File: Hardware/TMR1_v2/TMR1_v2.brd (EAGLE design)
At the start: 34.3 x 34.3 mm, 47 parts, among them U1 ATMEGA328P_TQFP, U2 MCP79410I/SN, Y1 32.768kHz

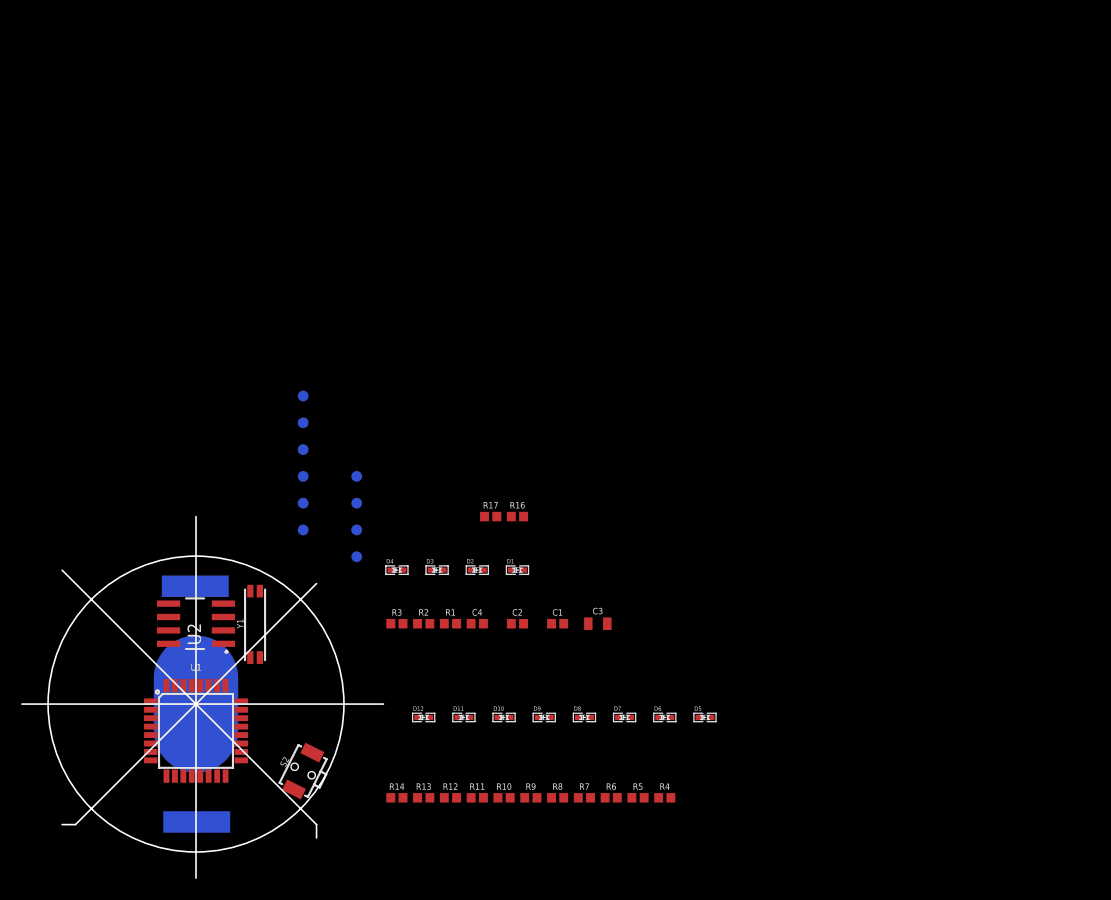
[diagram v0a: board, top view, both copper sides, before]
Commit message: std easy schematic with all elements in board before route
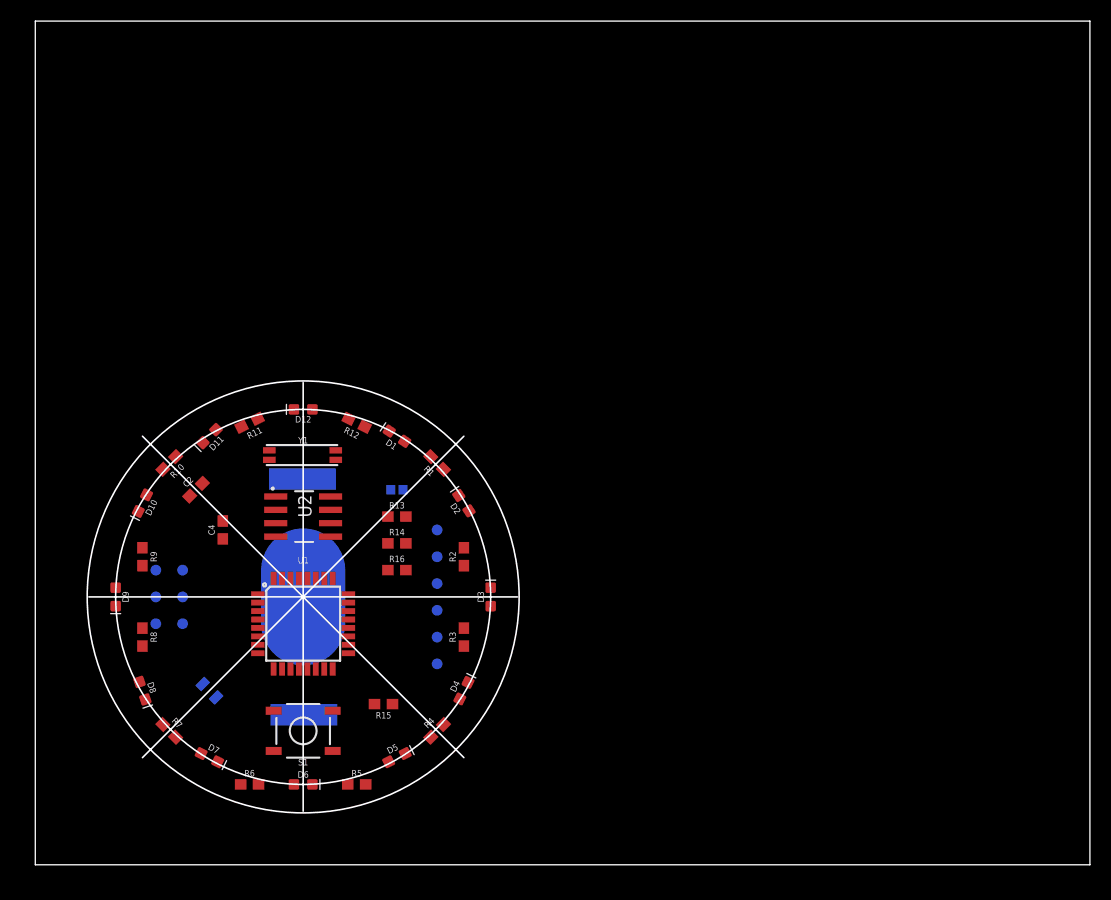
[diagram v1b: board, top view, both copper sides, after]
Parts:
- removed R17: 4.7k, SparkFun-Resistors:0402
- removed S2: MOMENTARY-SWITCH-SPST-SMD-RIGHT-ANGLE, SparkFun-Switches:TACTILE_SWITCH_SMD_RIGHT_ANGLE
- added R15: 10k, SparkFun-Resistors:0603
- added S1: MOMENTARY-SWITCH-SPST-SMD-5.2MM, SparkFun-Switches:TACTILE_SWITCH_SMD_5.2MM
- added TP11, TP12: TEST-POINT3X4, SparkFun-Connectors:PAD.03X.04
- C2, C4: value 6.8pF -> 22pF; device SparkFun-Capacitors:0402 -> SparkFun-Capacitors:0603
- C3: value 10uF -> 100nF
- D1, D10, D11, D12, D2, D3, D4, D5, D6, D7, D8, D9: device standardparts:0402.LED -> SparkFun-LED:LED-0603
- R1, R10, R11, R12, R2, R3, R4, R5, R6, R7, R8, R9: value 200 -> 330; device SparkFun-Resistors:0402 -> SparkFun-Resistors:0603
- R13, R14: device SparkFun-Resistors:0402 -> SparkFun-Resistors:0603
- R16: value 4.7k -> 10k; device SparkFun-Resistors:0402 -> SparkFun-Resistors:0603
- moved R10 44.9 mm to (12.7, 38.1), turned to 225 degrees
- moved R9 43.3 mm to (10.2, 29.2), turned to 270 degrees
- moved D9 42.2 mm to (7.62, 25.4), turned to 270 degrees
- moved R8 42.2 mm to (10.2, 21.6), turned to 270 degrees
- moved D8 42.0 mm to (10.2, 16.5), turned to 288.5 degrees
- moved R11 41.6 mm to (20.3, 41.9), turned to 206.5 degrees
- moved R7 39.9 mm to (12.7, 12.7), turned to 315 degrees
- moved D10 39.9 mm to (10.2, 34.3), turned to 243.5 degrees
- moved D7 39.6 mm to (16.5, 10.2), turned to 333.5 degrees
- moved C3 37.4 mm to (16.5, 16.5), flipped to the bottom, turned to 225 degrees
- moved R12 36.7 mm to (30.5, 41.9), turned to 153.5 degrees
- moved D11 36.0 mm to (16.5, 40.6), turned to 225 degrees
- moved D6 34.9 mm to (25.4, 7.62)
- moved R6 34.3 mm to (20.3, 7.62)
- moved C2 33.0 mm to (15.2, 35.6), turned to 45 degrees
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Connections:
- net D1: now also R1.1; no longer R1.2
- net D10: now also R10.1; no longer R10.2
- net D11: now also R11.1; no longer R11.2
- net D12: now also R12.1; no longer R12.2
- net D2: now also R2.1; no longer R2.2
- net D3: now also R3.1; no longer R3.2
- net D4: now also R4.1; no longer R4.2
- net D5: now also R5.1; no longer R5.2
- net D6: now also R6.1; no longer R6.2
- net D7: now also R7.1; no longer R7.2
- net D8: now also R8.1; no longer R8.2
- net D9: now also R9.1; no longer R9.2
- net GND: now also C2.1, C4.1, D1.C, D10.C, D11.C, D12.C, D2.C, D3.C, D4.C, D5.C, D6.C, D7.C, D8.C, D9.C, R15.1, TP12.P$1; no longer C2.2, C4.2, D1.P$2, D10.P$2, D11.P$2, D12.P$2, D2.P$2, D3.P$2, D4.P$2, D5.P$2, D6.P$2, D7.P$2, D8.P$2, D9.P$2, R14.2
- net MISO: now also TP7.P$1; no longer TP8.P$1
- net MOSI: now also TP10.P$1; no longer TP9.P$1
- net N$1: now also D8.A, R8.2; no longer D8.P$1, R8.1
- net N$10: now also C4.2; no longer C2.1
- net N$18: now also D9.A, R9.2; no longer D9.P$1, R9.1
- net N$2: now also D7.A, R7.2; no longer D7.P$1, R7.1
- net N$20: now also D10.A, R10.2; no longer D10.P$1, R10.1
- net N$22: now also D11.A, R11.2; no longer D11.P$1, R11.1
- net N$24: now also D12.A, R12.2; no longer D12.P$1, R12.1
- net N$3: now also D6.A, R6.2; no longer D6.P$1, R6.1
- net N$4: now also D5.A, R5.2; no longer D5.P$1, R5.1
- net N$5: now also D4.A, R4.2; no longer D4.P$1, R4.1
- net N$6: now also D3.A, R3.2; no longer D3.P$1, R3.1
- net N$7: now also D2.A, R2.2; no longer D2.P$1, R2.1
- net N$8: now also D1.A, R1.2; no longer D1.P$1, R1.1
- net N$9: now also C2.2; no longer C4.1
- net PUSH: now also R15.2, S1.3; no longer R14.1, S2.2
- net RST: now also R16.1, TP11.P$1; no longer R13.2, TP10.P$1
- net SCK: now also TP9.P$1; no longer TP7.P$1
- net SCL: now also R13.1; no longer R17.2
- net SDA: now also R14.1; no longer R16.2
- net VCC: now also R13.2, R14.2, R16.2, S1.1, TP8.P$1; no longer R13.1, R16.1, R17.1, S2.1
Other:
- board size 34.3 x 34.3 mm -> 100 x 80 mm
